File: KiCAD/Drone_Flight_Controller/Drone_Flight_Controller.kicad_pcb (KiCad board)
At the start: 2 copper layers, 83 x 45.1 mm, 107 parts, among them J201 Conn_01x04, J205 XT60, J207 Conn_01x05, P601 USB_C_Plug_USB2.0, Q201 BC846C, Q202 BC856C, Q203 BC846C, Q204 BC856C, Q205 BC846C, Q206 BC856C, Q207 BC846C, Q208 BC856C, Q401 2N2222A, Q601 BC846C, Q602 BC846C, Q603 BC846C, Q604 BC846C, Q605 BC846C, Q606 BC846C, Q607 BC846C, U201 AS358, U202 AS358, U205 AS358, U301 DPS368, U302 BNO055, U303 ESP32-WROOM-32, U601 MCP2200-I-SO, U701 LM2576-3.3WT, Y601 CSTNE12M0GH5L000R0

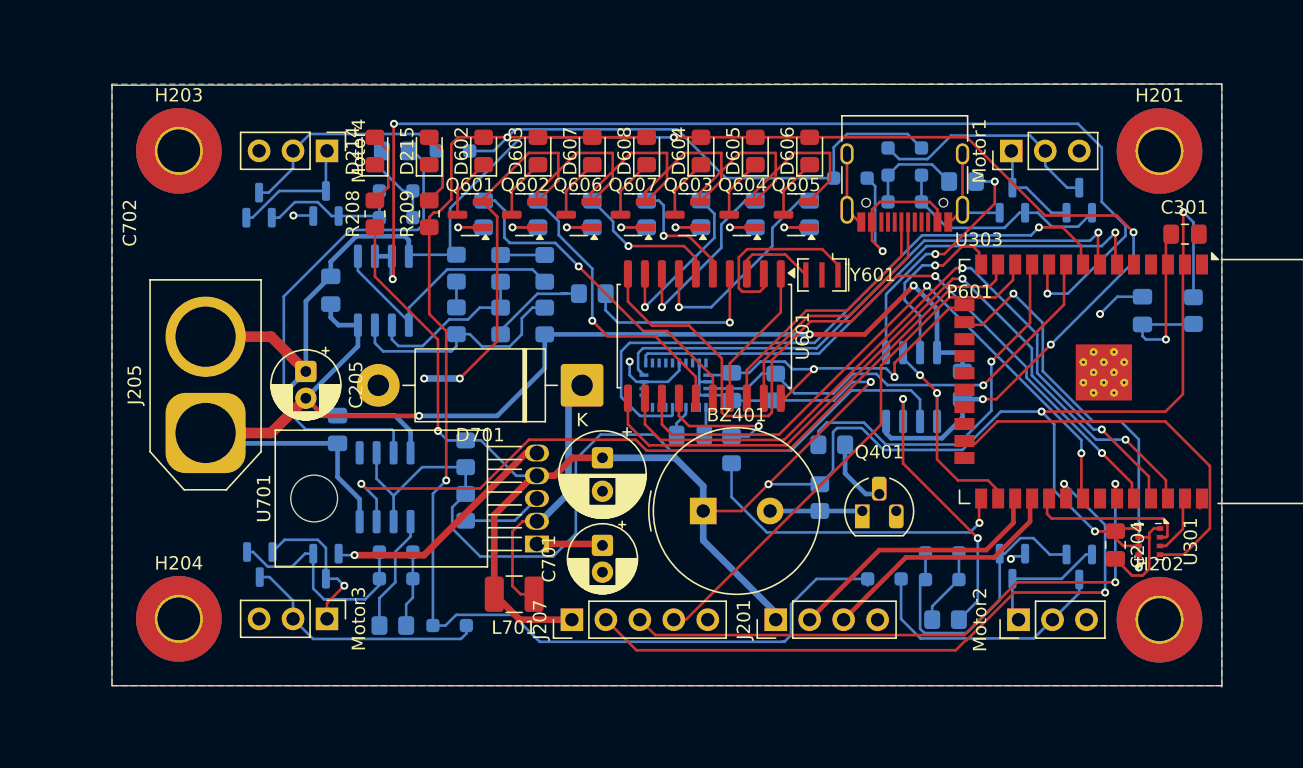
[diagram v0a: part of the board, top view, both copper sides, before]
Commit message: extend board length
extend board length
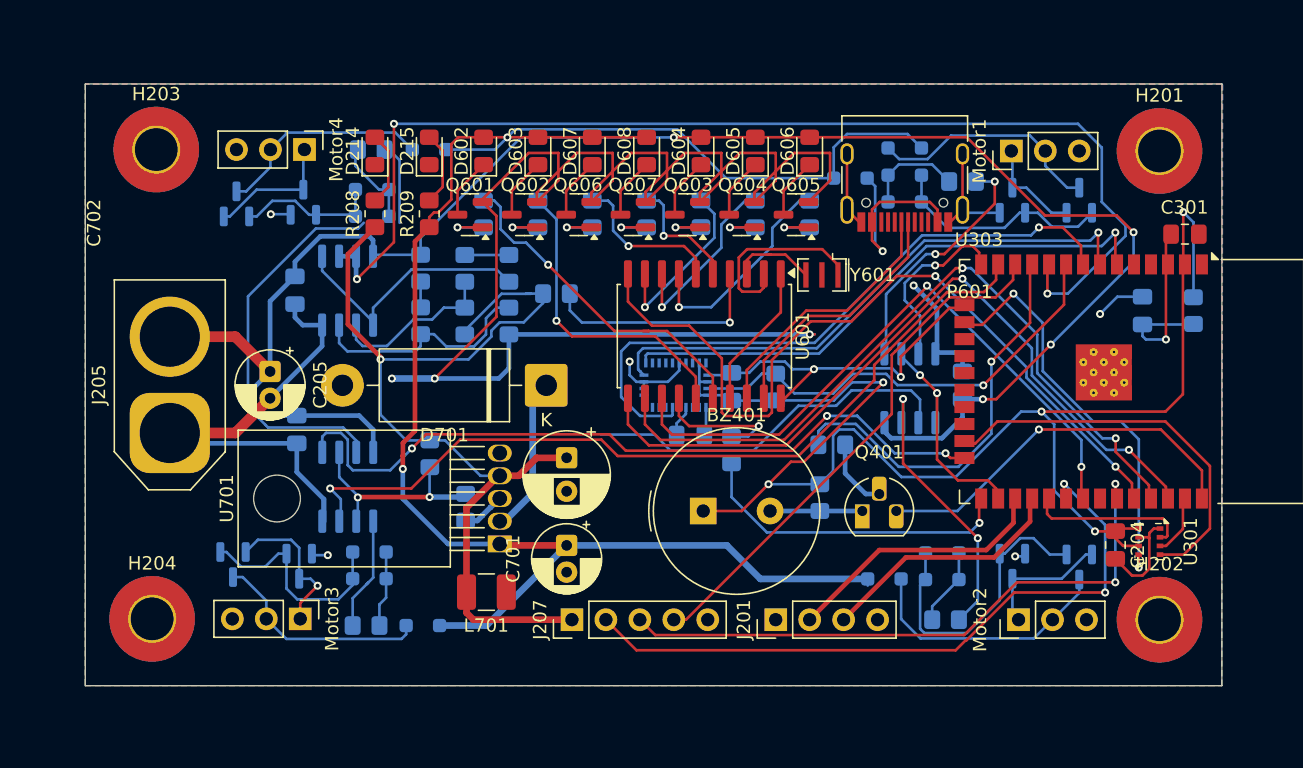
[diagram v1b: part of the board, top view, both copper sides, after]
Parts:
- moved C209 3.05 mm to (83.8, 100.8)
- moved U202 2.79 mm to (87.6, 105.1)
- moved U701 2.78 mm to (99.0, 109.4)
- moved C701 2.68 mm to (104.0, 109.5)
- moved C702 2.68 mm to (104.0, 103.0)
- moved C205 2.68 mm to (81.8, 96.5)
- moved C210 2.68 mm to (83.7, 90.4)
- moved D701 2.68 mm to (102.5, 97.5)
- moved J205 2.68 mm to (74.3, 101.1)
- moved R202 2.68 mm to (93.8, 102.7)
- moved R501 2.68 mm to (99.7, 92.7)
- moved R502 2.68 mm to (93.1, 88.8)
- moved R503 2.68 mm to (93.1, 92.7)
- moved R504 2.68 mm to (96.4, 92.7)
- moved R505 2.68 mm to (96.4, 88.8)
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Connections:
- C205 pad 2: -BATT -> GND
- C206 pad 2: -BATT -> GND
- C207 pad 2: -BATT -> GND
- C208 pad 2: -BATT -> GND
- C209 pad 2: -BATT -> GND
- C210 pad 2: -BATT -> GND
- C701 pad 1: 4V76 -> +4V76
- J205 pad 1: -BATT -> GND
- R501 pad 2: -BATT -> GND
- U201 pad 4: -BATT -> GND
- U202 pad 4: -BATT -> GND
- U205 pad 4: -BATT -> GND
- U701 pad 1: 4V76 -> +4V76
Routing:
- net -BATT: track 99.1 -> 0.00 mm, vias 3 -> 0
- net GND: track 176.2 -> 265.5 mm, vias 9 -> 12
- net Motor4: track 0.00 -> 55.6 mm, vias 0 -> 3
- net +1V7: track 64.1 -> 44.2 mm, vias 0 -> 2
- net Net-(D701-K): track 19.8 -> 11.7 mm
- net 4V76: track 5.05 -> 0.00 mm
- net +4V76: track 129.2 -> 133.6 mm
- net Motor3: track 59.0 -> 62.1 mm
- net Net-(U601-RST): track 14.5 -> 17.2 mm
- net Net-(D207-A): track 18.9 -> 16.5 mm
- net Net-(R206-Pad1): track 38.1 -> 35.8 mm
- net Buzzer: track 27.9 -> 30.2 mm
- net Net-(Q601-B): track 1.83 -> 3.78 mm
- net Net-(U601-GP1/USB-CFG): track 21.8 -> 23.3 mm
- net BATT Monitor: track 85.3 -> 86.5 mm
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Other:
- board size 83 x 45.1 mm -> 85 x 45 mm
